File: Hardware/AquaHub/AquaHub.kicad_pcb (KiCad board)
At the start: 2 copper layers, 198.1 x 118.7 mm, 43 parts, among them J1 Screw_Terminal, J10 PinHeader4, J11 PinHeader3, J12 PinHeader3, J2 Screw_Terminal, J3 Screw_Terminal, J4 Screw_Terminal, J5 Screw_Terminal, J6 Screw_Terminal, J7 Screw_Terminal, J8 Screw_Terminal, J9 PinHeader3, K1 MT2-C93402, K2 MT2-C93402, K3 MT2-C93402, K4 MT2-C93402, K5 MT2-C93402, K6 MT2-C93402, U1 ESP32-WROVER-I, U2 ACS723, U3 3.3V Reg, U4 TPL7407LA, U5 5V Reg

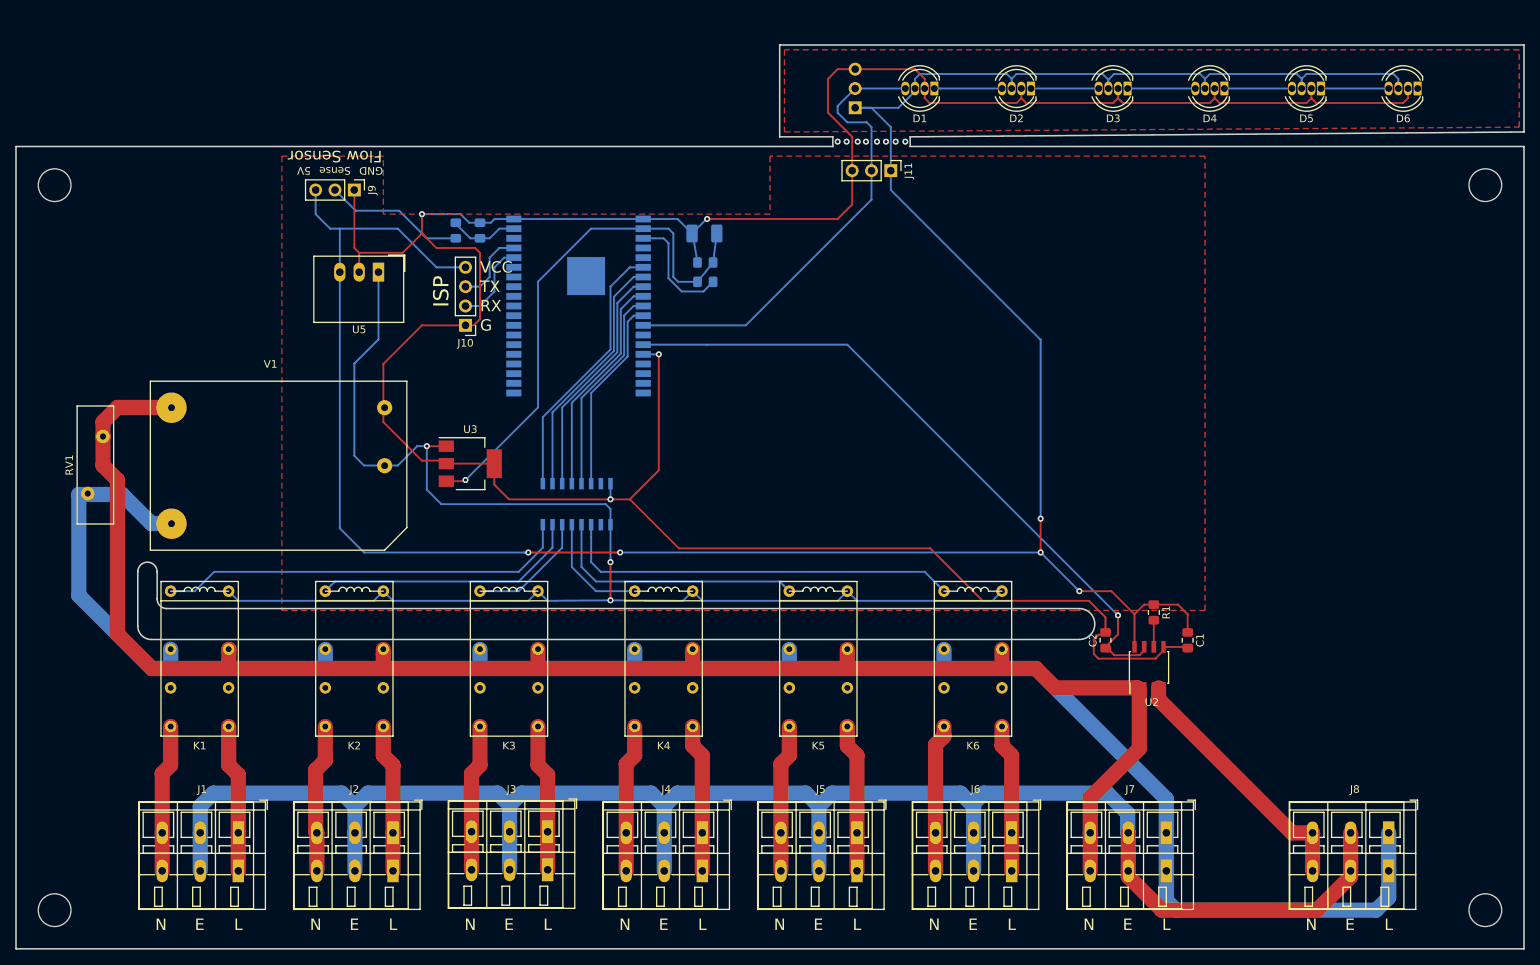
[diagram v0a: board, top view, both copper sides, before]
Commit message: Lots of new stuff
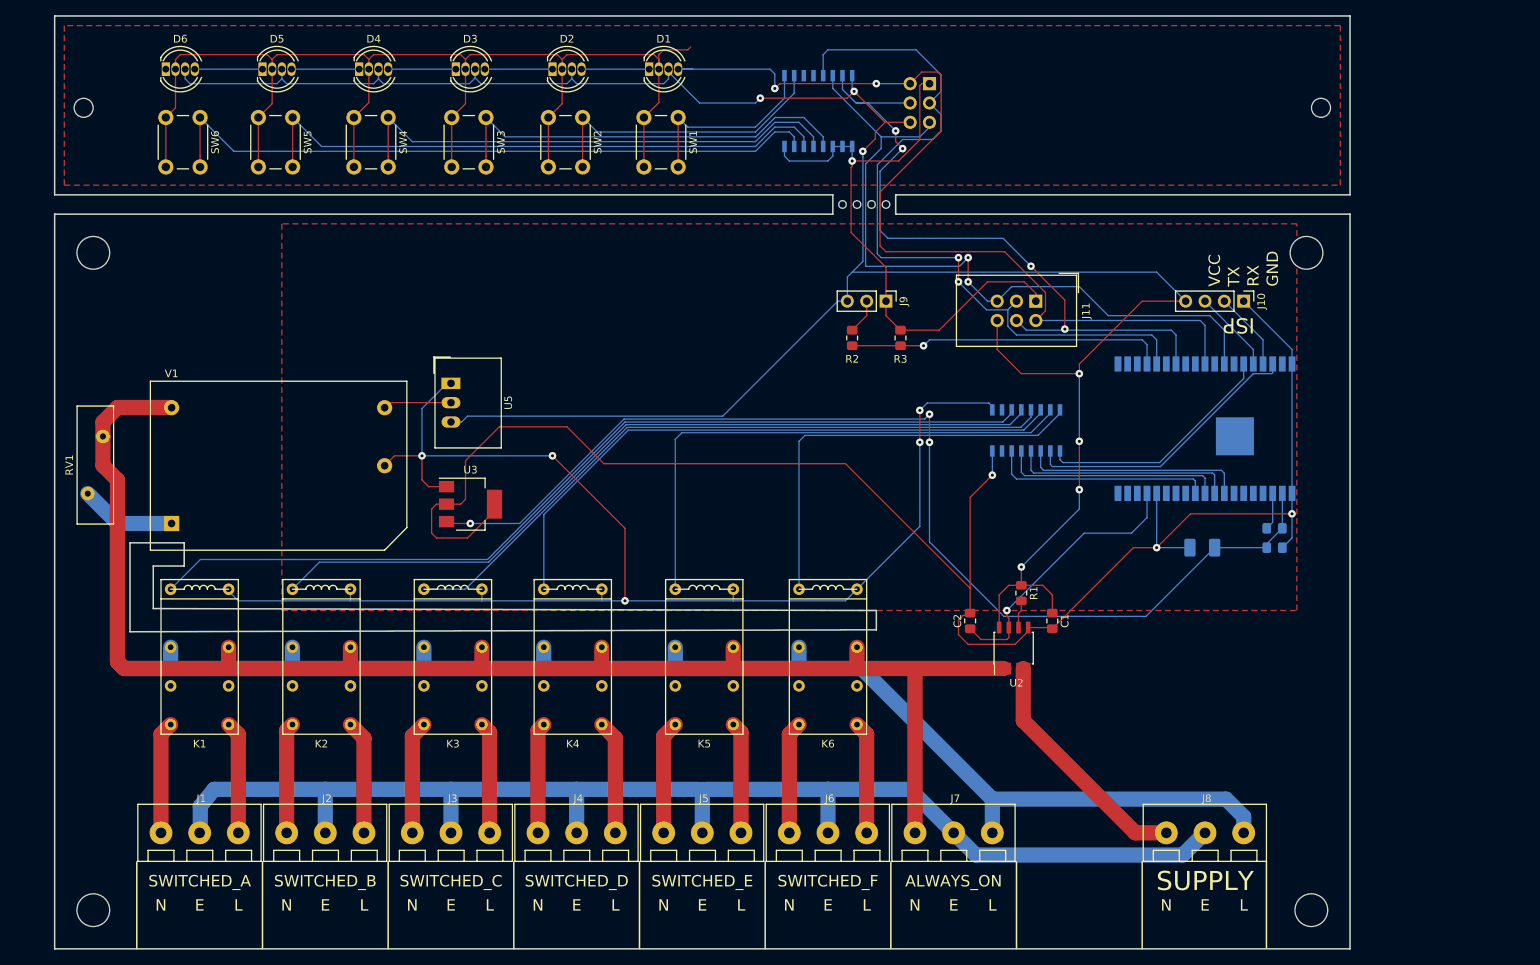
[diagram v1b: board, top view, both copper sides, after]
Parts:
- added MH10: MountingHole, AquaFootprints:Breakaway 1mm, F.Cu at (141.6, 62.2)
- added MH5: MountingHole, MountingHole:MountingHole_2.5mm, F.Cu at (204.5, 49.5)
- added MH6: MountingHole, MountingHole:MountingHole_2.5mm, F.Cu at (41.9, 49.5)
- added MH7: MountingHole, AquaFootprints:Breakaway 1mm, F.Cu at (147.3, 62.2)
- added MH8: MountingHole, AquaFootprints:Breakaway 1mm, F.Cu at (145.4, 62.2)
- added MH9: MountingHole, AquaFootprints:Breakaway 1mm, F.Cu at (143.5, 62.2)
- added SW1: SW_Push, Button_Switch_THT:SW_PUSH_6mm_H13mm, F.Cu at (120.0, 50.8)
- added SW2: SW_Push, Button_Switch_THT:SW_PUSH_6mm_H13mm, F.Cu at (107.5, 50.8)
- added SW3: SW_Push, Button_Switch_THT:SW_PUSH_6mm_H13mm, F.Cu at (94.8, 50.8)
- added SW4: SW_Push, Button_Switch_THT:SW_PUSH_6mm_H13mm, F.Cu at (81.9, 50.8)
- added SW5: SW_Push, Button_Switch_THT:SW_PUSH_6mm_H13mm, F.Cu at (69.4, 50.8)
- added SW6: SW_Push, Button_Switch_THT:SW_PUSH_6mm_H13mm, F.Cu at (57.2, 50.8)
- added U6: TCA9534, Package_SO:SOIC-16W_7.5x12.8mm_P1.27mm, B.Cu at (138.4, 50.0)
- D1, D2, D3, D4, D5, D6: footprint LED_THT:LED_D5.0mm-4 -> LED_THT:LED_D5.0mm-4_RGB
- J1, J2, J3, J4, J5, J6, J7, J8: footprint TerminalBlock_WAGO:TerminalBlock_WAGO_236-103_1x03_P5.00mm_45Degree -> AquaFootprints:weidmuller_pm-5.08-3-way
- J11, J12: value PinHeader3 -> Conn_01x06; footprint Connector_PinHeader_2.54mm:PinHeader_1x03_P2.54mm_Vertical -> Connector_IDC:IDC-Header_2x03_P2.54mm_Vertical
- R2, R3: moved to F.Cu
- U1: value ESP32-WROVER-I -> ESP32-WROVER; footprint AquaFootprints:ESP32-WROVER -> Module:Espressif_ESP32_WROVER
- V1: footprint AquaFootprints:RAC01-GB -> Converter_ACDC:Converter_ACDC_RECOM_RAC01-xxSGB_THT
- moved D6 164.5 mm to (52.7, 44.5), turned to 0 degrees
- moved D5 139.1 mm to (65.4, 44.5), turned to 0 degrees
- moved D4 113.7 mm to (78.1, 44.5), turned to 0 degrees
- moved J10 102.3 mm to (194.3, 74.9), turned to 270 degrees
- moved D3 88.3 mm to (90.8, 44.5), turned to 0 degrees
- moved C3 83.6 mm to (198.4, 107.3), turned to 0 degrees
- moved R4 81.5 mm to (198.4, 104.8), turned to 0 degrees
- moved C4 77.3 mm to (188.9, 107.3)
- moved U1 73.4 mm to (189.2, 91.7), turned to 90 degrees
- moved J9 71.4 mm to (147.3, 74.9)
- moved D2 62.9 mm to (103.5, 44.5), turned to 0 degrees
- moved U4 59.8 mm to (165.7, 91.9), turned to 90 degrees
- moved R3 57.0 mm to (149.2, 79.8)
- moved R2 53.9 mm to (142.9, 79.8), turned to 90 degrees
- moved D1 37.6 mm to (116.2, 44.5), turned to 0 degrees
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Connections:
- net POW3 renamed /POW3
- net POW4 renamed /POW4
- net POW5 renamed /POW5
- net POW6 renamed /POW6
- D1 pad 4: PANEL_LEDS -> /Panel_LED
- J1 pad 1: LIVE1 -> NEUTRAL1
- J1 pad 3: NEUTRAL1 -> LIVE1
- J10 pad 2: RX -> TX
- J10 pad 3: TX -> RX
- J11 pad 1: +5V -> GND
- J11 pad 2: PANEL_LEDS -> /Panel_LED
- J11 pad 3: GND -> /Panel_INT
- J12 pad 1: +5V -> GND
- J12 pad 2: PANEL_LEDS -> /Panel_LED
- J12 pad 3: GND -> /Panel_INT
- J2 pad 1: LIVE2 -> NEUTRAL2
- J2 pad 3: NEUTRAL2 -> LIVE2
- J3 pad 1: LIVE3 -> NEUTRAL3
- J3 pad 3: NEUTRAL3 -> LIVE3
- J4 pad 1: LIVE4 -> NEUTRAL4
- J4 pad 3: NEUTRAL4 -> LIVE4
- J5 pad 1: LIVE5 -> NEUTRAL5
- J5 pad 3: NEUTRAL5 -> LIVE5
- J6 pad 1: LIVE6 -> NEUTRAL6
- J6 pad 3: NEUTRAL6 -> LIVE6
- J7 pad 1: NEUTRAL -> LIVE
- J7 pad 3: LIVE -> NEUTRAL
- J8 pad 1: NEUTRAL -> /LIVE_IN
- J8 pad 3: /LIVE_IN -> NEUTRAL
- R2 pad 1: FLOW_SENSE -> /FLOW_SENSE
- R3 pad 2: FLOW_SENSE -> /FLOW_SENSE
- U1 pad 12: PANEL_LEDS -> (no net)
- U1 pad 14: POWER_SENSE -> (no net)
- U1 pad 16: (no net) -> POWER_SENSE
- U1 pad 23: (no net) -> /FLOW_SENSE
- U1 pad 24: (no net) -> /Panel_INT
- U1 pad 26: (no net) -> /Panel_SDA
- U1 pad 29: (no net) -> /Panel_LED
- U1 pad 31: (no net) -> /Panel_SCL
- U1 pad 33: (no net) -> /POW1
- U1 pad 36: (no net) -> /POW2
- U1 pad 37: FLOW_SENSE -> (no net)
- U1 pad 6: POW1 -> (no net)
- U1 pad 7: POW2 -> (no net)
- U4 pad 1: POW1 -> /POW1
- U4 pad 11: RE6 -> RE1
- U4 pad 12: RE5 -> RE2
- U4 pad 13: RE4 -> RE3
- U4 pad 14: RE3 -> RE4
- U4 pad 15: RE2 -> RE5
- U4 pad 16: RE1 -> RE6
- U4 pad 2: POW2 -> /POW2
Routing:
- net /Panel_LED: track 0.00 -> 121.5 mm, vias 0 -> 2
- net /Panel_INT: track 0.00 -> 99.7 mm, vias 0 -> 2
- net /Panel_SCL: track 0.00 -> 95.5 mm, vias 0 -> 2
- net GND: track 384.4 -> 476.5 mm
- net /Panel_SDA: track 0.00 -> 90.3 mm, vias 0 -> 4
- net Net-(SW6-Pad1): track 0.00 -> 89.0 mm
- net Net-(SW5-Pad1): track 0.00 -> 78.1 mm
- net +3V3: track 69.8 -> 146.3 mm, vias 1 -> 3
- net RE3: track 16.2 -> 90.1 mm
- net RE2: track 35.2 -> 106.5 mm
- net Net-(SW4-Pad1): track 0.00 -> 67.3 mm
- net RE1: track 54.3 -> 120.5 mm
- net RE4: track 15.1 -> 81.0 mm
- net PANEL_LEDS: track 62.3 -> 0.00 mm
- net EARTH: track 228.8 -> 169.0 mm
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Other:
- board size 198.1 x 118.7 mm -> 170.2 x 122.6 mm
- net class Default: trace_width 0.25 -> 0.1524; via_dia 0.8 -> 1
- net class MainsRails: via_dia 0.8 -> 1
- rule via_min_size: 0.4 -> 1
- board text added: "ALWAYS_ON"
- board text added: "SUPPLY"
- board text added: "SWITCHED_A"
- board text added: "SWITCHED_B"
- board text added: "SWITCHED_C"
- board text added: "SWITCHED_D"
- board text added: "SWITCHED_E"
- board text added: "SWITCHED_F"
- board text removed: "5V"
- board text removed: "Flow Sensor"
- board text removed: "G"
- board text removed: "Sense"
